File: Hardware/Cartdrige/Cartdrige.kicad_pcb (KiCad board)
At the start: 2 copper layers, 80 x 34.3 mm, 4 parts, among them J1 ROM, U1 28C256

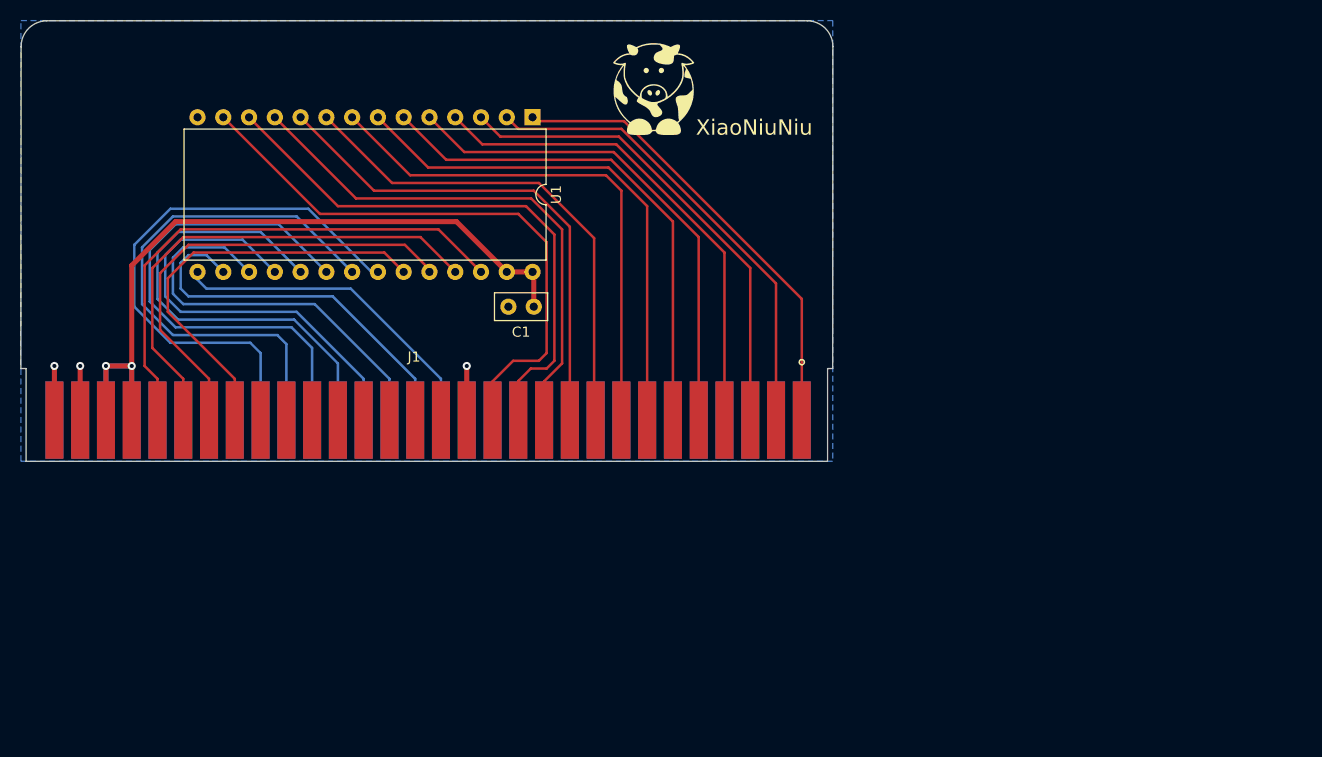
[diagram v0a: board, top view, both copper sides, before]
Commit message: Finalize 1.3
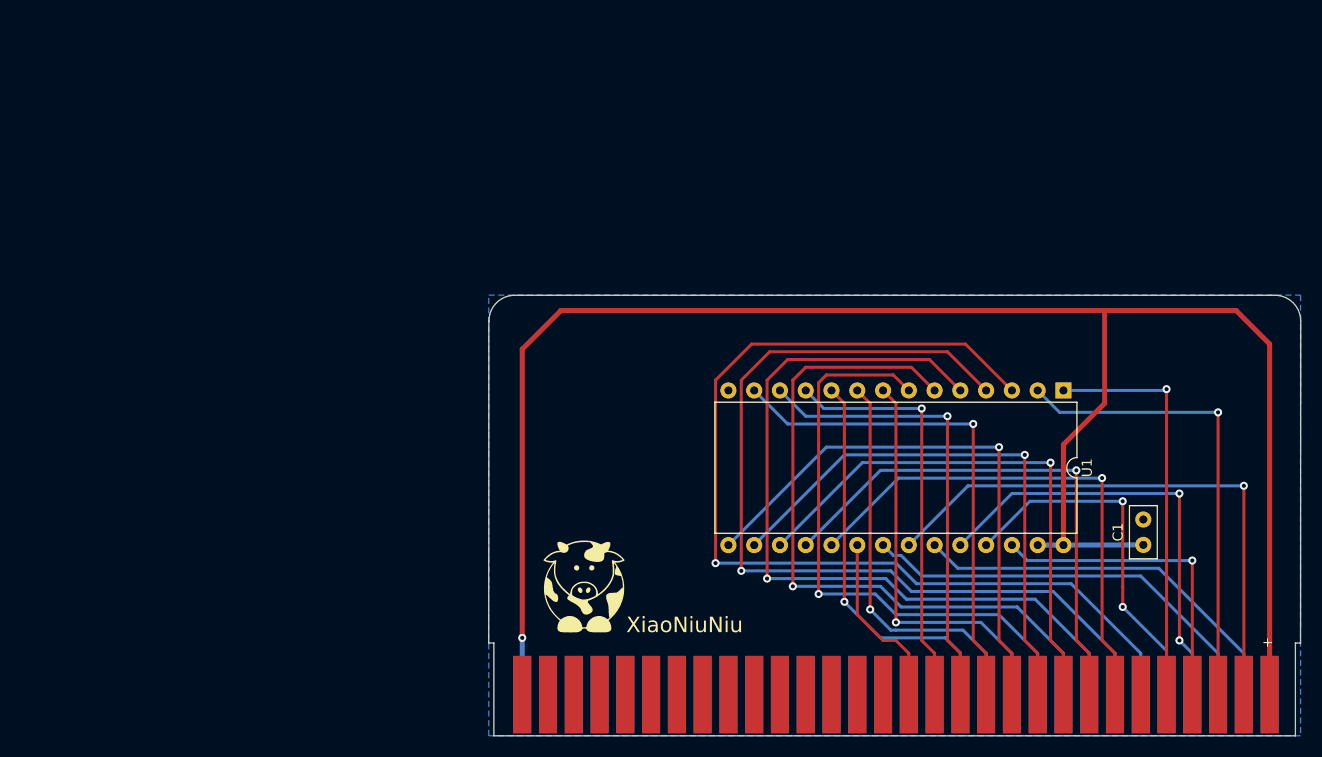
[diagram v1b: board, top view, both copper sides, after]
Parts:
- removed J1: ROM, Connector_TheRLab:NES_PCBEdge
- removed the XiaoNiuNiu at (87.9, 32.0)
- added J2: PORT1, NESConnector:NES_PCBEdge, F.Cu at (110.5, 91.7)
- added XiaoNiuNiu: LOGO, Cow:VerySmallCow, F.Cu at (81.0, 81.0)
- moved C1 64.5 mm to (136.1, 76.9), turned to 90 degrees
- moved U1 58.8 mm to (128.3, 61.7)
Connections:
- U1 pad 20: CS -> /PORT1CSB
- U1 pad 22: OE -> /CLOCK
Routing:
- net +5V: track 83.3 -> 180.4 mm, vias 2 -> 1
- net /CLOCK: track 0.00 -> 56.0 mm, vias 0 -> 1
- net OE: track 55.1 -> 0.00 mm
- net /A7: track 47.7 -> 100.3 mm, vias 0 -> 1
- net CS: track 50.5 -> 0.00 mm
- net /A6: track 48.6 -> 89.9 mm, vias 0 -> 1
- net /A5: track 49.5 -> 79.6 mm, vias 0 -> 1
- net /D3: track 32.9 -> 55.6 mm, vias 0 -> 1
- net /A13: track 52.1 -> 31.6 mm, vias 0 -> 1
- net /A4: track 50.4 -> 69.2 mm, vias 0 -> 1
- net /PORT1CSB: track 0.00 -> 17.6 mm
- net GND: track 16.0 -> 0.00 mm, vias 3 -> 0
- net /D4: track 38.6 -> 54.5 mm, vias 0 -> 1
- net /A8: track 48.8 -> 36.1 mm, vias 0 -> 2
- net /D5: track 41.3 -> 53.4 mm, vias 0 -> 1
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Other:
- board text added: "+"
